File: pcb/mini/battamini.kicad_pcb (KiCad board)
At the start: 2 copper layers, 128.3 x 99.3 mm, 38 parts

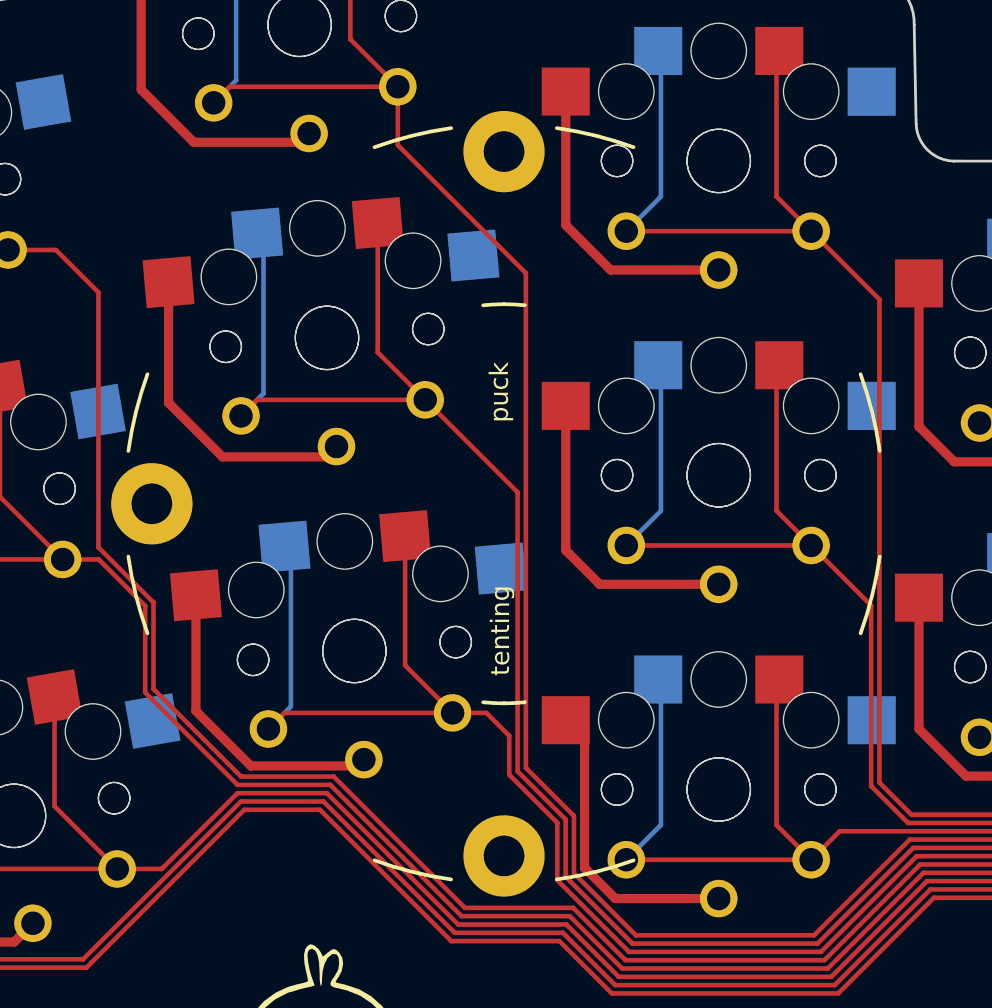
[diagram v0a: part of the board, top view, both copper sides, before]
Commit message: updated gerber
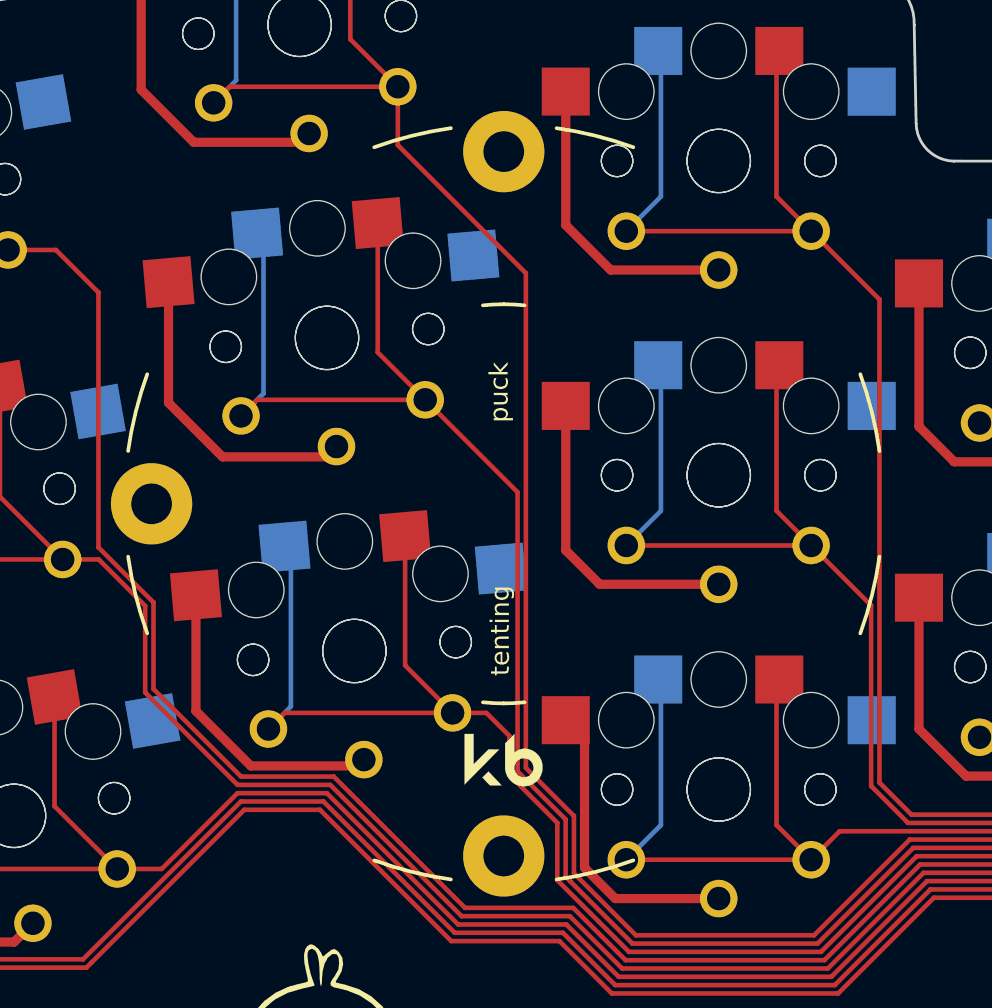
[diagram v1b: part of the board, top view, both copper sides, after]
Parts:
- removed the REF** at (103.8, -88.1)
- added REF**: Tenting Puck, kbd:Tenting_Puck2, F.Cu at (103.8, -88.1)
